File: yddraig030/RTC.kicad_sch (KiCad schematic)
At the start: 11 parts, among them Q1301 BC549B, Q1302 2N4403, U1301 RTC-72421

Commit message: Working on PCB layout
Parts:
- C1301, C1302: footprint Capacitor_THT:C_Disc_D3.8mm_W2.6mm_P2.50mm -> Capacitor_SMD:C_0805_2012Metric
- C1303: footprint Capacitor_THT:CP_Radial_D5.0mm_P2.50mm -> Capacitor_SMD:CP_Elec_4x5.3
- D1301: footprint Diode_THT:D_DO-35_SOD27_P7.62mm_Horizontal -> Diode_SMD:D_SOD-123
- R1301, R1302, R1303: footprint Resistor_THT:R_Axial_DIN0207_L6.3mm_D2.5mm_P10.16mm_Horizontal -> Resistor_SMD:R_0805_2012Metric
- U1301: footprint Package_DIP:DIP-18_W7.62mm_Socket -> Package_SO:SOP-18_7x12.5mm_P1.27mm
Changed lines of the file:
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@@
     (property "Reference" "U1301" (id 0) (at 190.5 96.52 0))
     (property "Value" "RTC-72421" (id 1) (at 191.77 127 0))
-    (property "Footprint" "Package_DIP:DIP-18_W7.62mm_Socket" (id 2) (at 181.61 109.22 0)
+    (property "Footprint" "Package_SO:SOP-18_7x12.5mm_P1.27mm" (id 2) (at 181.61 109.22 0)
       (effects (font (size 1.27 1.27)) hide)
     )
@@
       (effects (font (size 1.27 1.27)) (justify left))
     )
-    (property "Footprint" "Diode_THT:D_DO-35_SOD27_P7.62mm_Horizontal" (id 2) (at 99.695 82.55 0)
+    (property "Footprint" "Diode_SMD:D_SOD-123" (id 2) (at 99.695 82.55 0)
       (effects (font (size 1.27 1.27)) hide)
     )
@@
       (effects (font (size 1.27 1.27)) (justify left))
     )
-    (property "Footprint" "Resistor_THT:R_Axial_DIN0207_L6.3mm_D2.5mm_P10.16mm_Horizontal" (id 2) (at 70.612 106.68 90)
+    (property "Footprint" "Resistor_SMD:R_0805_2012Metric" (id 2) (at 70.612 106.68 90)
       (effects (font (size 1.27 1.27)) hide)
     )
@@
       (effects (font (size 1.27 1.27)) (justify left))
     )
-    (property "Footprint" "Capacitor_THT:CP_Radial_D5.0mm_P2.50mm" (id 2) (at 121.6152 91.44 0)
+    (property "Footprint" "Capacitor_SMD:CP_Elec_4x5.3" (id 2) (at 121.6152 91.44 0)
       (effects (font (size 1.27 1.27)) hide)
     )
@@
       (effects (font (size 1.27 1.27)) (justify left))
     )
-    (property "Footprint" "Resistor_THT:R_Axial_DIN0207_L6.3mm_D2.5mm_P10.16mm_Horizontal" (id 2) (at 84.582 88.9 90)
+    (property "Footprint" "Resistor_SMD:R_0805_2012Metric" (id 2) (at 84.582 88.9 90)
       (effects (font (size 1.27 1.27)) hide)
     )
@@
       (effects (font (size 1.27 1.27)) (justify left))
     )
-    (property "Footprint" "Resistor_THT:R_Axial_DIN0207_L6.3mm_D2.5mm_P10.16mm_Horizontal" (id 2) (at 70.612 88.9 90)
+    (property "Footprint" "Resistor_SMD:R_0805_2012Metric" (id 2) (at 70.612 88.9 90)
       (effects (font (size 1.27 1.27)) hide)
     )
@@
       (effects (font (size 1.27 1.27)) (justify left))
     )
-    (property "Footprint" "Capacitor_THT:C_Disc_D3.8mm_W2.6mm_P2.50mm" (id 2) (at 114.5032 157.607 0)
+    (property "Footprint" "Capacitor_SMD:C_0805_2012Metric" (id 2) (at 114.5032 157.607 0)
       (effects (font (size 1.27 1.27)) hide)
     )
@@
       (effects (font (size 1.27 1.27)) (justify left))
     )
-    (property "Footprint" "Capacitor_THT:C_Disc_D3.8mm_W2.6mm_P2.50mm" (id 2) (at 102.4382 157.607 0)
-      (effects (font (size 1.27 1.27)) hide)
-    )
+    (property "Footprint" "Capacitor_SMD:C_0805_2012Metric" (id 2) (at 102.4382 157.607 0)
+      (effects (font (size 1.27 1.27)) hide)
+    )

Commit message: Some more changes to SMD version
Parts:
- U1301: footprint Package_SO:SOP-18_7x12.5mm_P1.27mm -> Package_DIP:DIP-18_W7.62mm_Socket
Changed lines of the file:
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@@
     (property "Reference" "U1301" (id 0) (at 190.5 96.52 0))
     (property "Value" "RTC-72421" (id 1) (at 191.77 127 0))
-    (property "Footprint" "Package_SO:SOP-18_7x12.5mm_P1.27mm" (id 2) (at 181.61 109.22 0)
+    (property "Footprint" "Package_DIP:DIP-18_W7.62mm_Socket" (id 2) (at 181.61 109.22 0)
       (effects (font (size 1.27 1.27)) hide)
     )

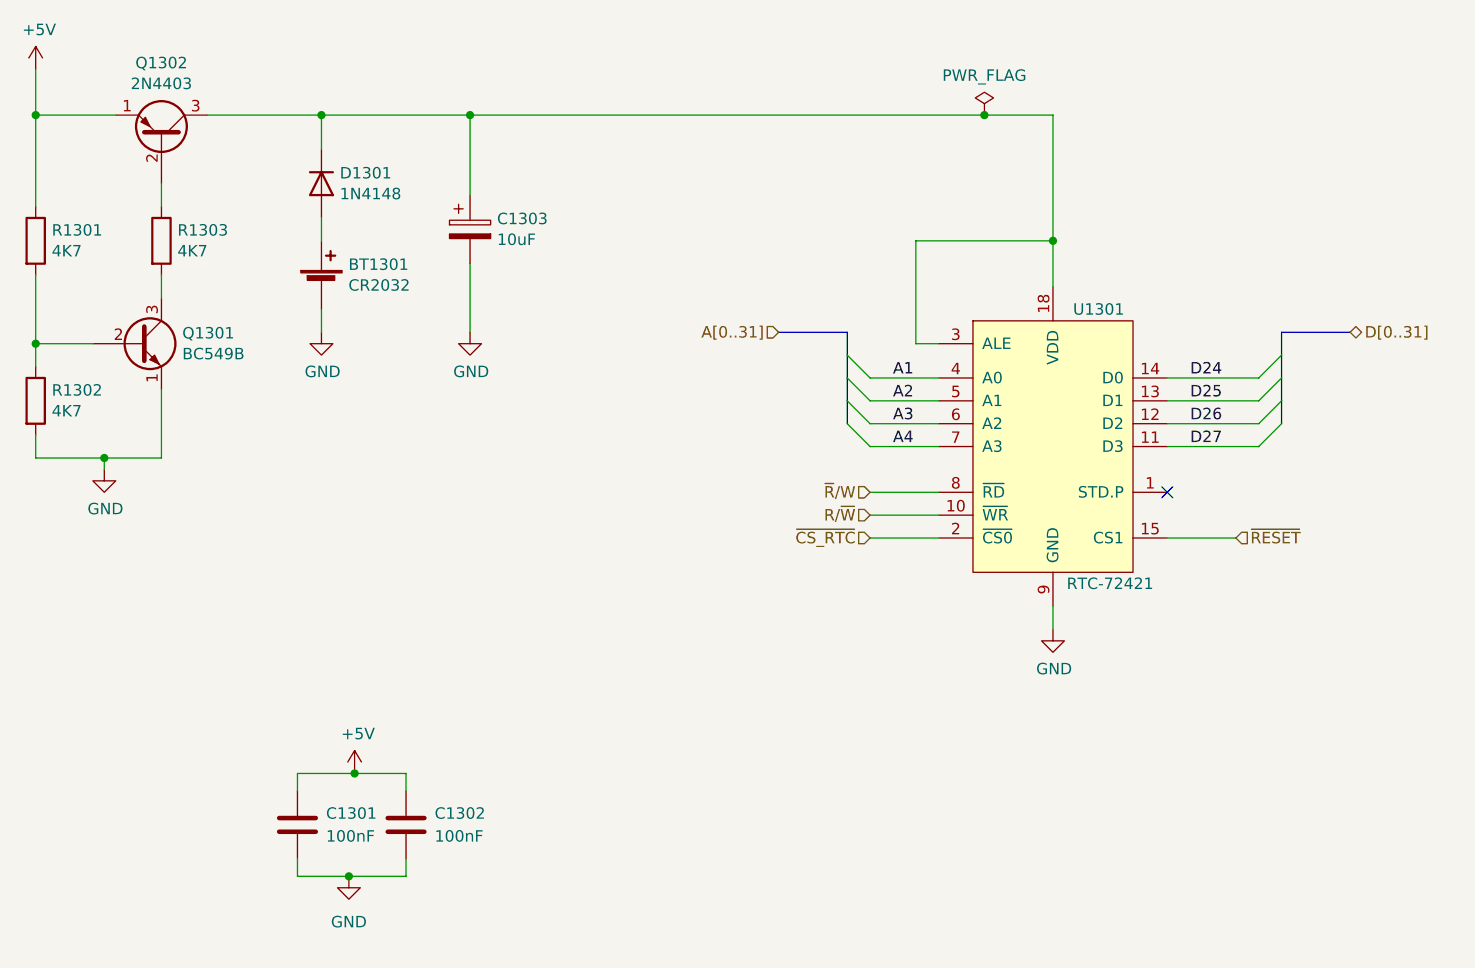
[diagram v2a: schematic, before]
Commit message: Cleaning up schematic and PCB
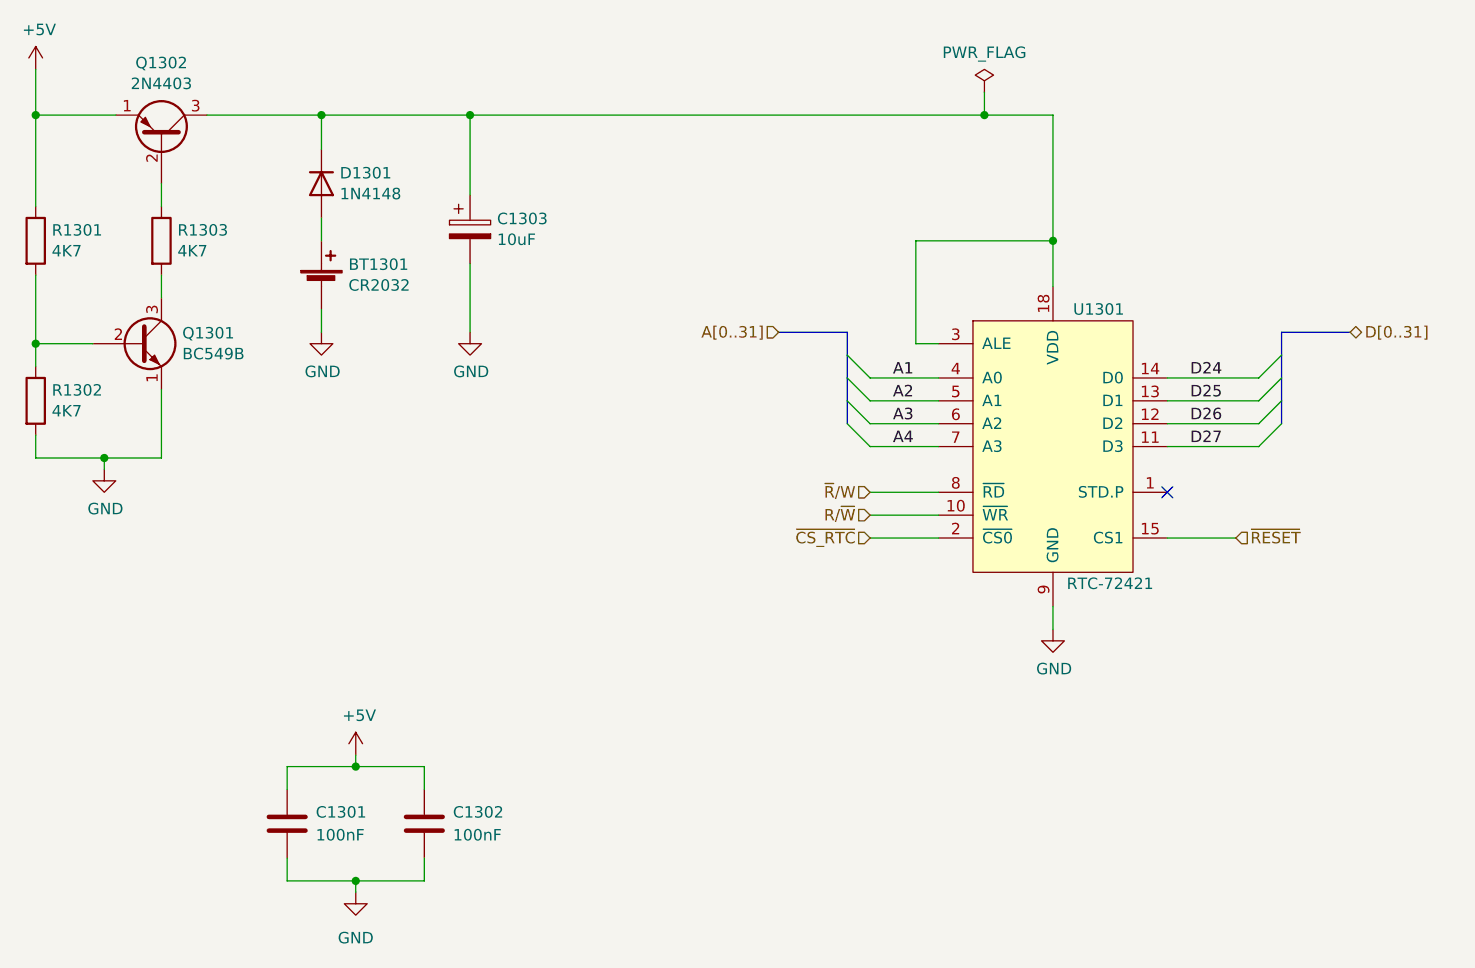
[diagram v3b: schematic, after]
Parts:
- D1301: footprint Diode_SMD:D_SOD-123 -> Diode_SMD:D_SOD-323
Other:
- moved on the sheet: C1301, C1302
